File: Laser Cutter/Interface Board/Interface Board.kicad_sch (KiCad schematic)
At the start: 93 parts, among them J1 Screw_Terminal_01x02, J10 Screw_Terminal_01x02, J11 Limit Switches Out, J12 Limit Switches Out, J2 Screw_Terminal_01x02, J3 Relay Signals, J4 Screw_Terminal_01x02, J5 Limit Switch X, J6 Limit Switches Out, J7 Limit Switch Y, J8 Door Switch, J9 Flow Sensor, K1 SANYOU_SRD_Form_C, K2 SANYOU_SRD_Form_C, U1 ULN2003, U2 74HC14, U3 L7805, U4 74HC14

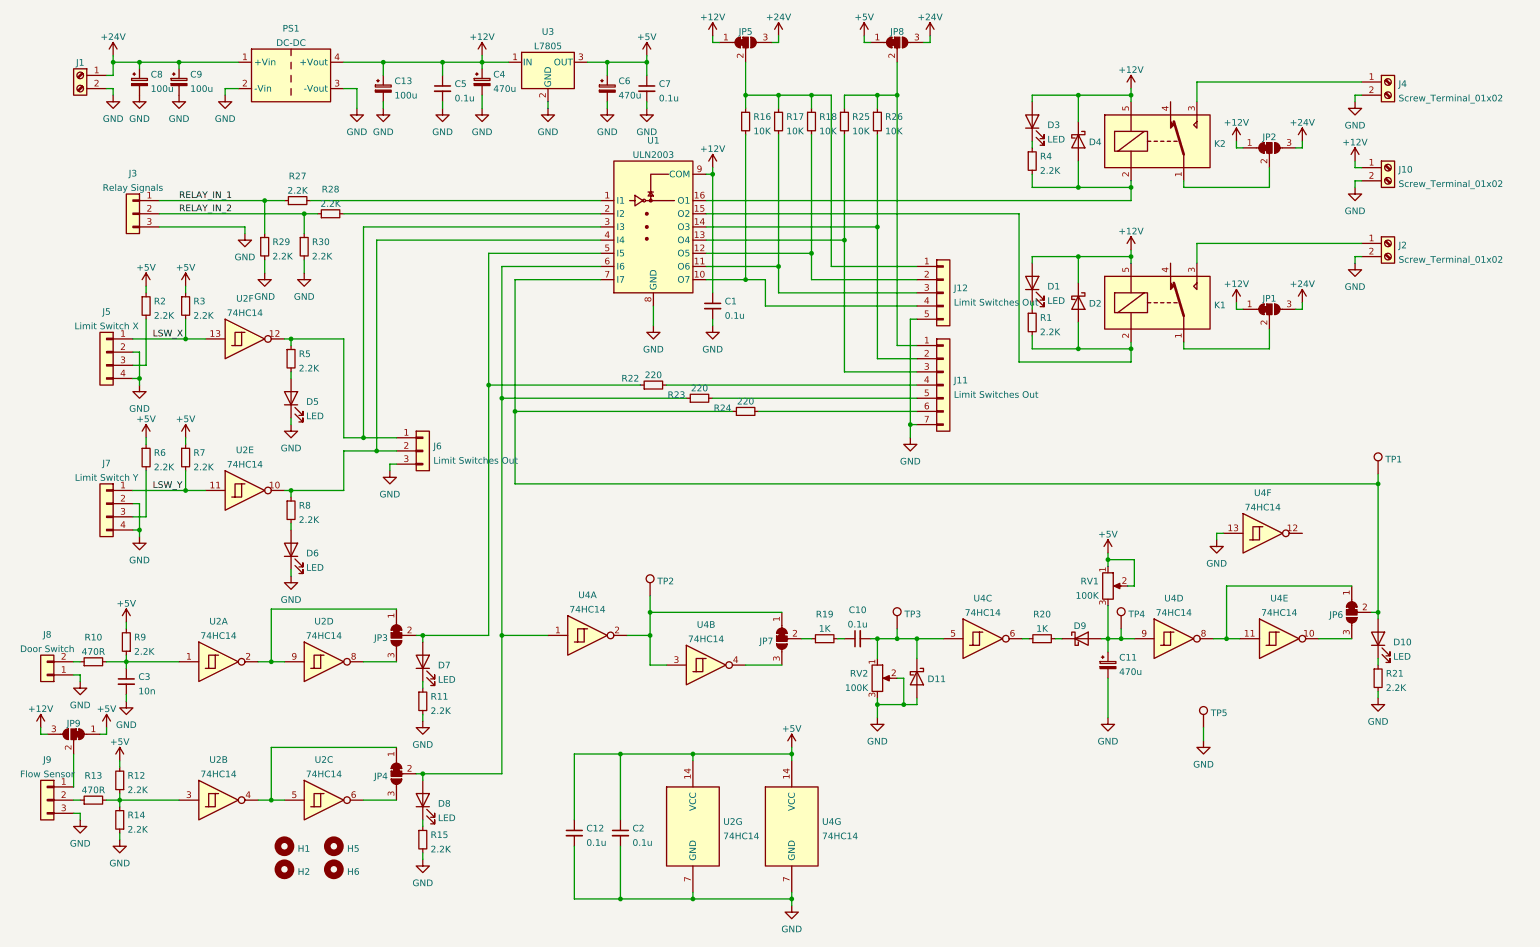
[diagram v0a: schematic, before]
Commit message: Blerp.
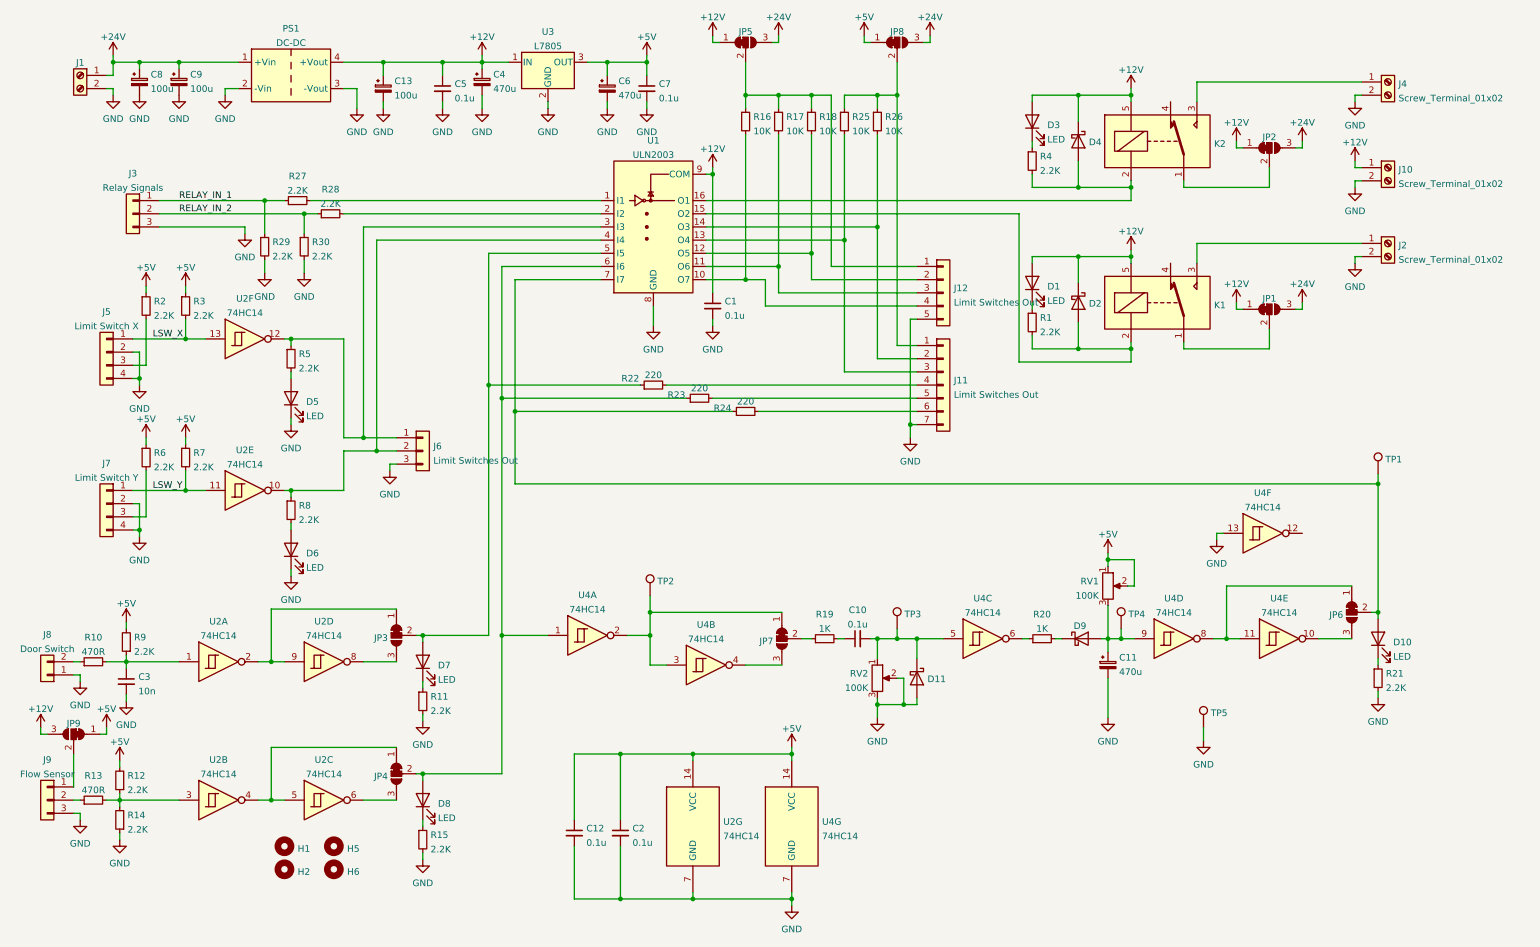
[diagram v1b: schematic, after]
